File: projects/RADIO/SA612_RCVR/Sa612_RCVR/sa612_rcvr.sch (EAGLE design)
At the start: 39 parts, among them IC1 SA612AN, Q1 BC238

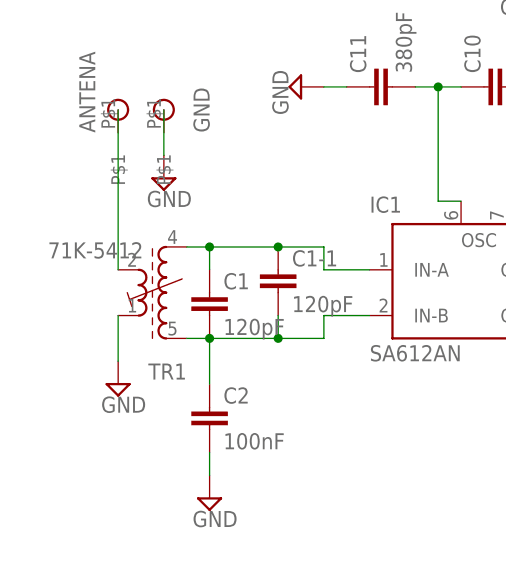
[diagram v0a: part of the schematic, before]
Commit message: update
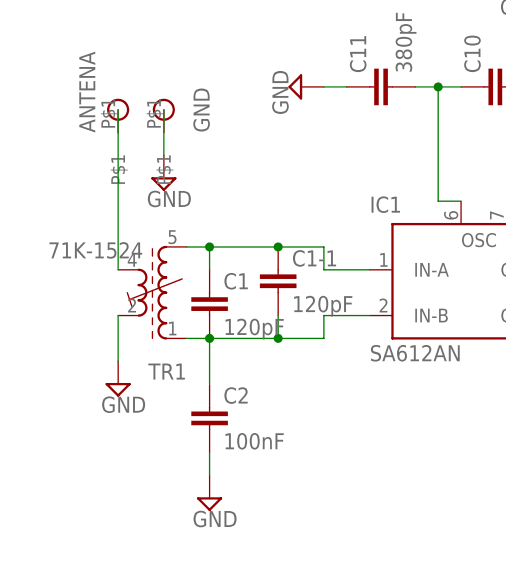
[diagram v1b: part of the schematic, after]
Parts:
- C7: device rcl:C-EU050-050X075 -> rcl:C-EU050-025X075
- TR1: value 71K-5412 -> 71K-1524; device inductor-neosid:71K-5412 -> inductor-neosid:71K-1524
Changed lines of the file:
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@@
 <parts>
 <part name="IC1" library="linear" library_urn="urn:adsk.eagle:library:262" deviceset="SA612A" device="N" package3d_urn="urn:adsk.eagle:package:16409/2"/>
-<part name="TR1" library="inductor-neosid" library_urn="urn:adsk.eagle:library:241" deviceset="71K-" device="5412" package3d_urn="urn:adsk.eagle:package:14718/1"/>
+<part name="TR1" library="inductor-neosid" deviceset="71K-" device="1524" package3d_urn="urn:adsk.eagle:package:14718/1"/>
 <part name="SUPPLY1" library="supply2" library_urn="urn:adsk.eagle:library:372" deviceset="GND" device=""/>
 <part name="SUPPLY2" library="supply2" library_urn="urn:adsk.eagle:library:372" deviceset="GND" device=""/>
@@
 <part name="R2" library="rcl" library_urn="urn:adsk.eagle:library:334" deviceset="R-EU_" device="R0805" package3d_urn="urn:adsk.eagle:package:23553/2" value="51*"/>
 <part name="R3" library="rcl" library_urn="urn:adsk.eagle:library:334" deviceset="R-EU_" device="R0805" package3d_urn="urn:adsk.eagle:package:23553/2" value="3.9k"/>
-<part name="C7" library="rcl" library_urn="urn:adsk.eagle:library:334" deviceset="C-EU" device="050-050X075" package3d_urn="urn:adsk.eagle:package:23665/1"/>
+<part name="C7" library="rcl" deviceset="C-EU" device="050-025X075" package3d_urn="urn:adsk.eagle:package:23637/1"/>
 <part name="R4" library="rcl" library_urn="urn:adsk.eagle:library:334" deviceset="R-TRIMM" device="64X" package3d_urn="urn:adsk.eagle:package:23749/1"/>
 <part name="SUPPLY7" library="supply2" library_urn="urn:adsk.eagle:library:372" deviceset="GND" device=""/>
@@
 <part name="U$8" library="mylib" deviceset="SMD_PIN" device=""/>
 <part name="SUPPLY17" library="supply2" library_urn="urn:adsk.eagle:library:372" deviceset="GND" device=""/>
-<part name="C1-1" library="rcl" library_urn="urn:adsk.eagle:library:334" deviceset="C-EU" device="050-025X075" package3d_urn="urn:adsk.eagle:package:23637/1" value="120pF"/>
+<part name="C1-1" library="rcl" deviceset="C-EU" device="050-025X075" package3d_urn="urn:adsk.eagle:package:23637/1" value="120pF"/>
 <part name="H1" library="holes" library_urn="urn:adsk.eagle:library:237" deviceset="MOUNT-PAD-ROUND" device="3.0" package3d_urn="urn:adsk.eagle:package:14280/1"/>
 <part name="H2" library="holes" library_urn="urn:adsk.eagle:library:237" deviceset="MOUNT-PAD-ROUND" device="3.0" package3d_urn="urn:adsk.eagle:package:14280/1"/>
